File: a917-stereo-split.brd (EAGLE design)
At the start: 100 x 26 mm, 38 parts, among them U1 SCREW-M2X8, U10 FX2-20S-1.27DS, U2 SCREW-M2X8, U3 NUT-M2-SELFLOCK, U4 NUT-M2-SELFLOCK, U5 FX2-20P-1.27DS, U6 SCREW-M2X8, U7 SCREW-M2X8, U8 NUT-M2-SELFLOCK, U9 NUT-M2-SELFLOCK

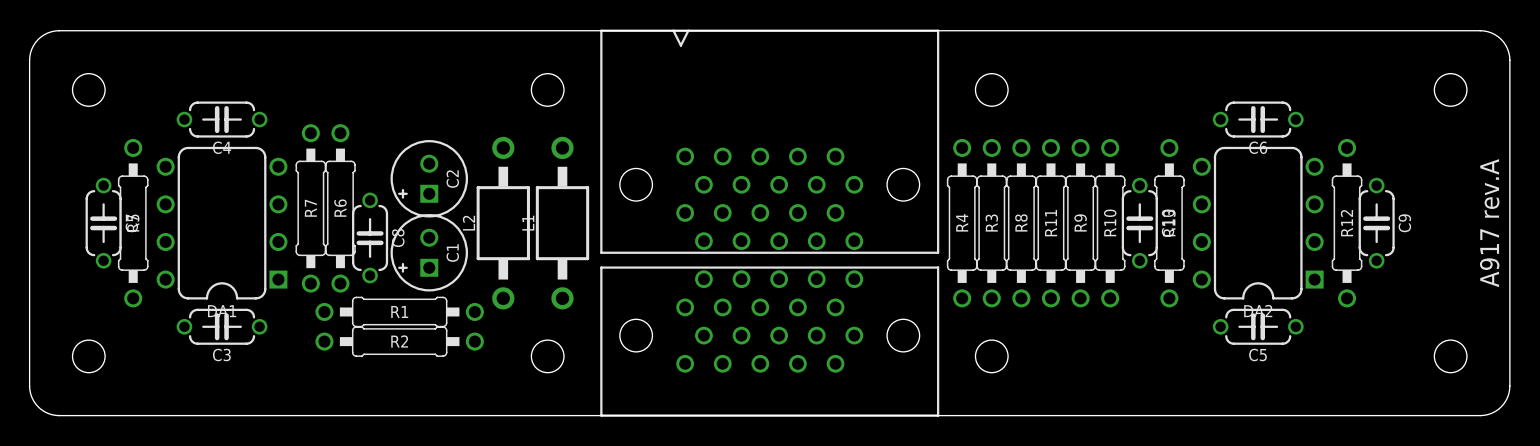
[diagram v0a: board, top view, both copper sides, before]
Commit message: A917 Routing
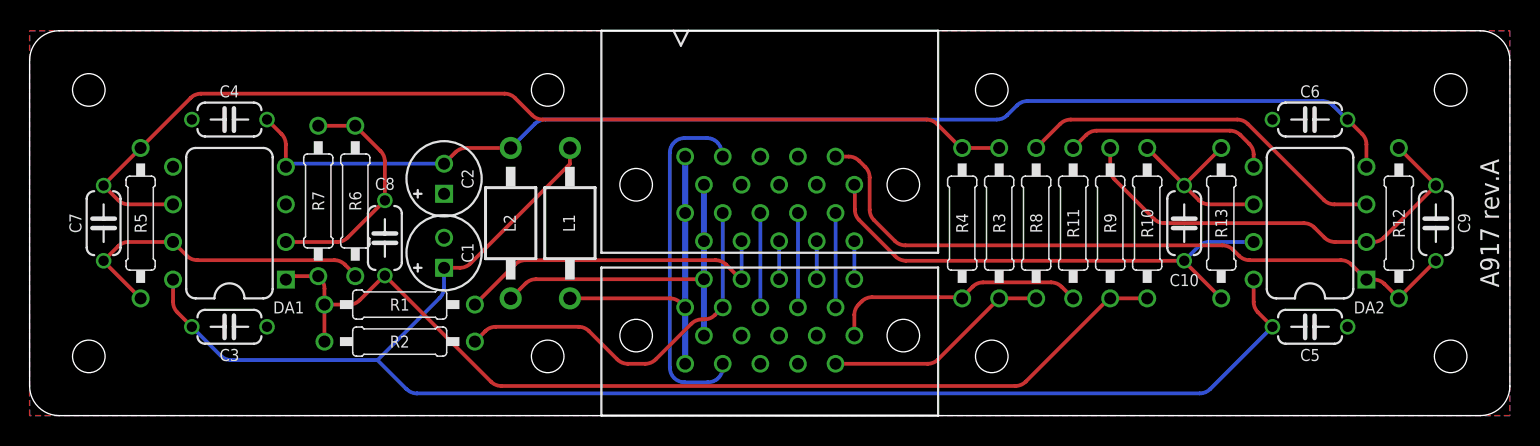
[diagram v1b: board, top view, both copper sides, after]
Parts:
- moved C9 4.00 mm to (95.0, 13.0)
- moved C5 3.50 mm to (86.5, 6.00)
- moved C6 3.50 mm to (86.5, 20.0)
- moved DA2 3.50 mm to (86.5, 13.0)
- moved R12 3.50 mm to (92.5, 13.0)
- moved R13 3.50 mm to (80.5, 13.0)
- moved C10 3.00 mm to (78.0, 13.0)
- moved R10 2.50 mm to (75.5, 13.0)
- moved R9 2.00 mm to (73.0, 13.0)
- moved R11 1.50 mm to (70.5, 13.0)
- moved R6 1.12 mm to (22.0, 14.5)
- moved C1 1.00 mm to (28.0, 11.0)
- moved C2 1.00 mm to (28.0, 16.0)
- moved C8 1.00 mm to (24.0, 12.0)
- moved R8 1.00 mm to (68.0, 13.0)
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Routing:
- net N$45: track 0.00 -> 104.3 mm
- net N$47: track 0.00 -> 81.1 mm
- net N$10: track 0.00 -> 69.5 mm
- net MONO: track 0.00 -> 68.5 mm
- net N$16: track 0.00 -> 46.9 mm
- net N$19: track 0.00 -> 34.2 mm
- net N$15: track 0.00 -> 30.5 mm
- net N$3: track 0.00 -> 25.8 mm
- net N$14: track 0.00 -> 25.3 mm
- net N$7: track 0.00 -> 23.8 mm
- net N$46: track 0.00 -> 23.7 mm
- net N$4: track 0.00 -> 22.2 mm
- net N$25: track 0.00 -> 22.0 mm
- net N$11: track 0.00 -> 21.9 mm
- net N$22: track 0.00 -> 17.6 mm
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- added copper zone on layer 1, net GND
- added copper zone on layer 16, net GND
